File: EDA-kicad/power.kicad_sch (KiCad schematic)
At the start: 93 parts, among them SW1 EG25-switch-CSS-1210MC, SW2 MIC-switch-CSS-1210MC, SW3 CAM-switch-CSS-1210MC, U10 22V-boost-AP3032KTR-G1, U11 MP3429GL-Z, U7 BQ25792RQMR, U8 TPS65023BRSBR, U9 BAT-CONNECTOR-FLTS22WR00

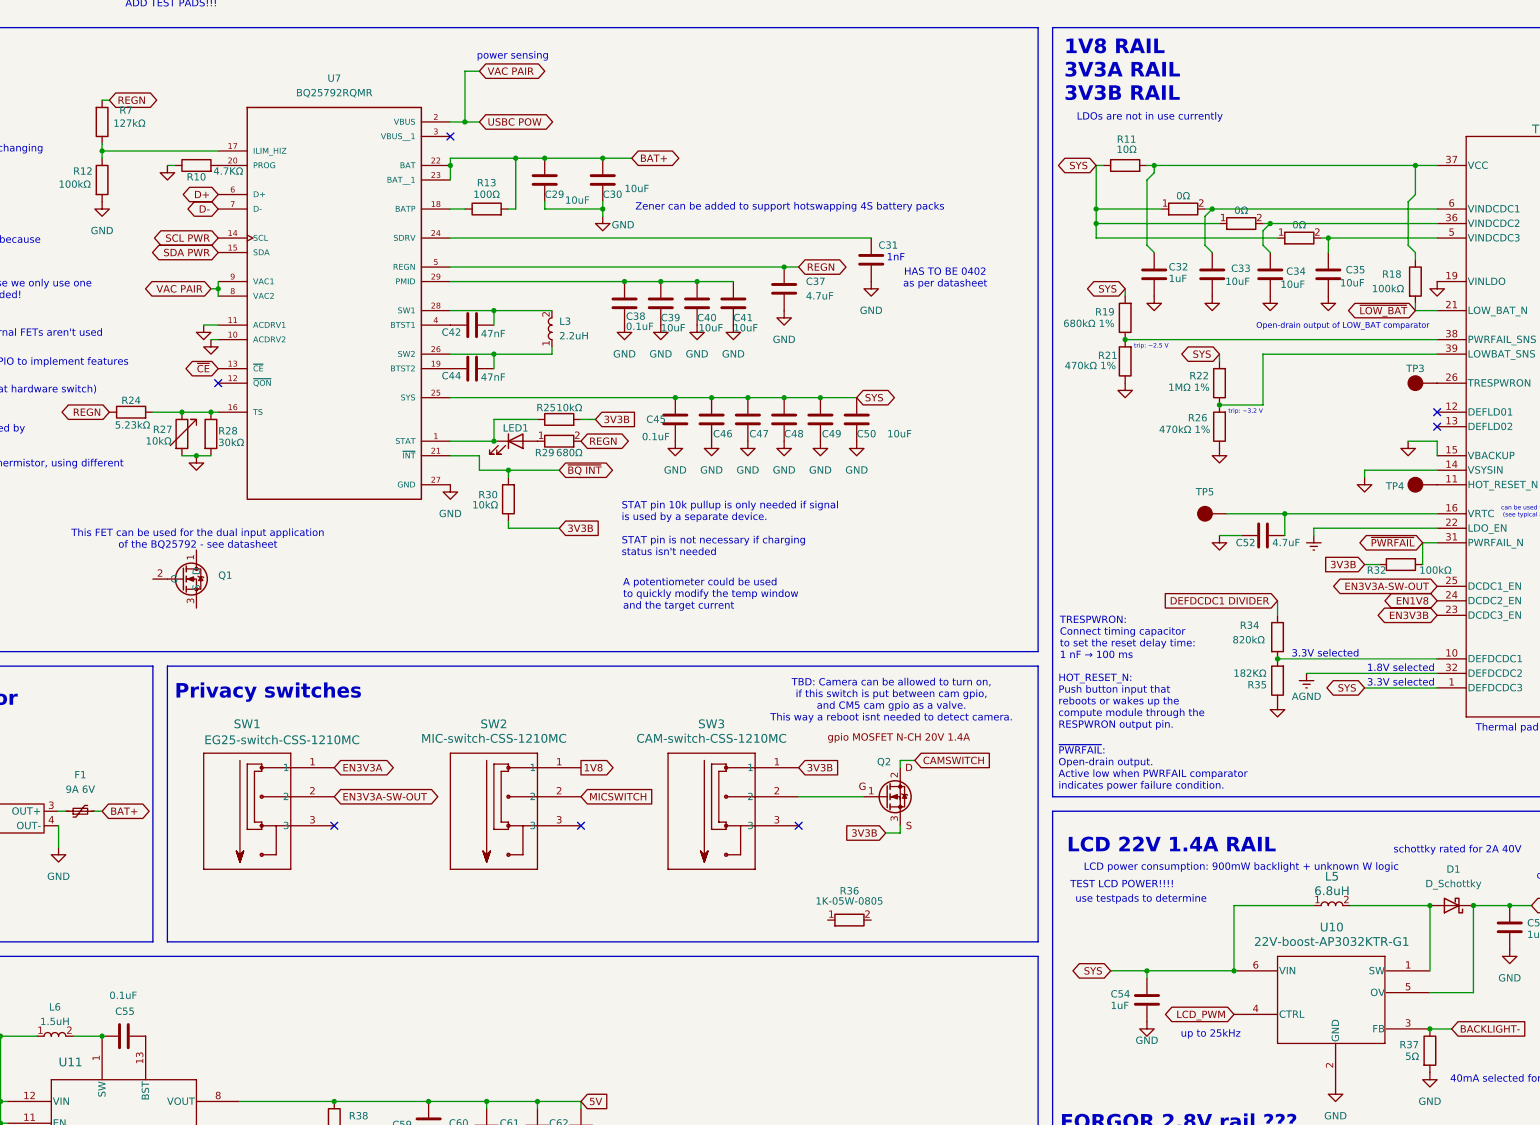
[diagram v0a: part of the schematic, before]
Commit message: change some labels
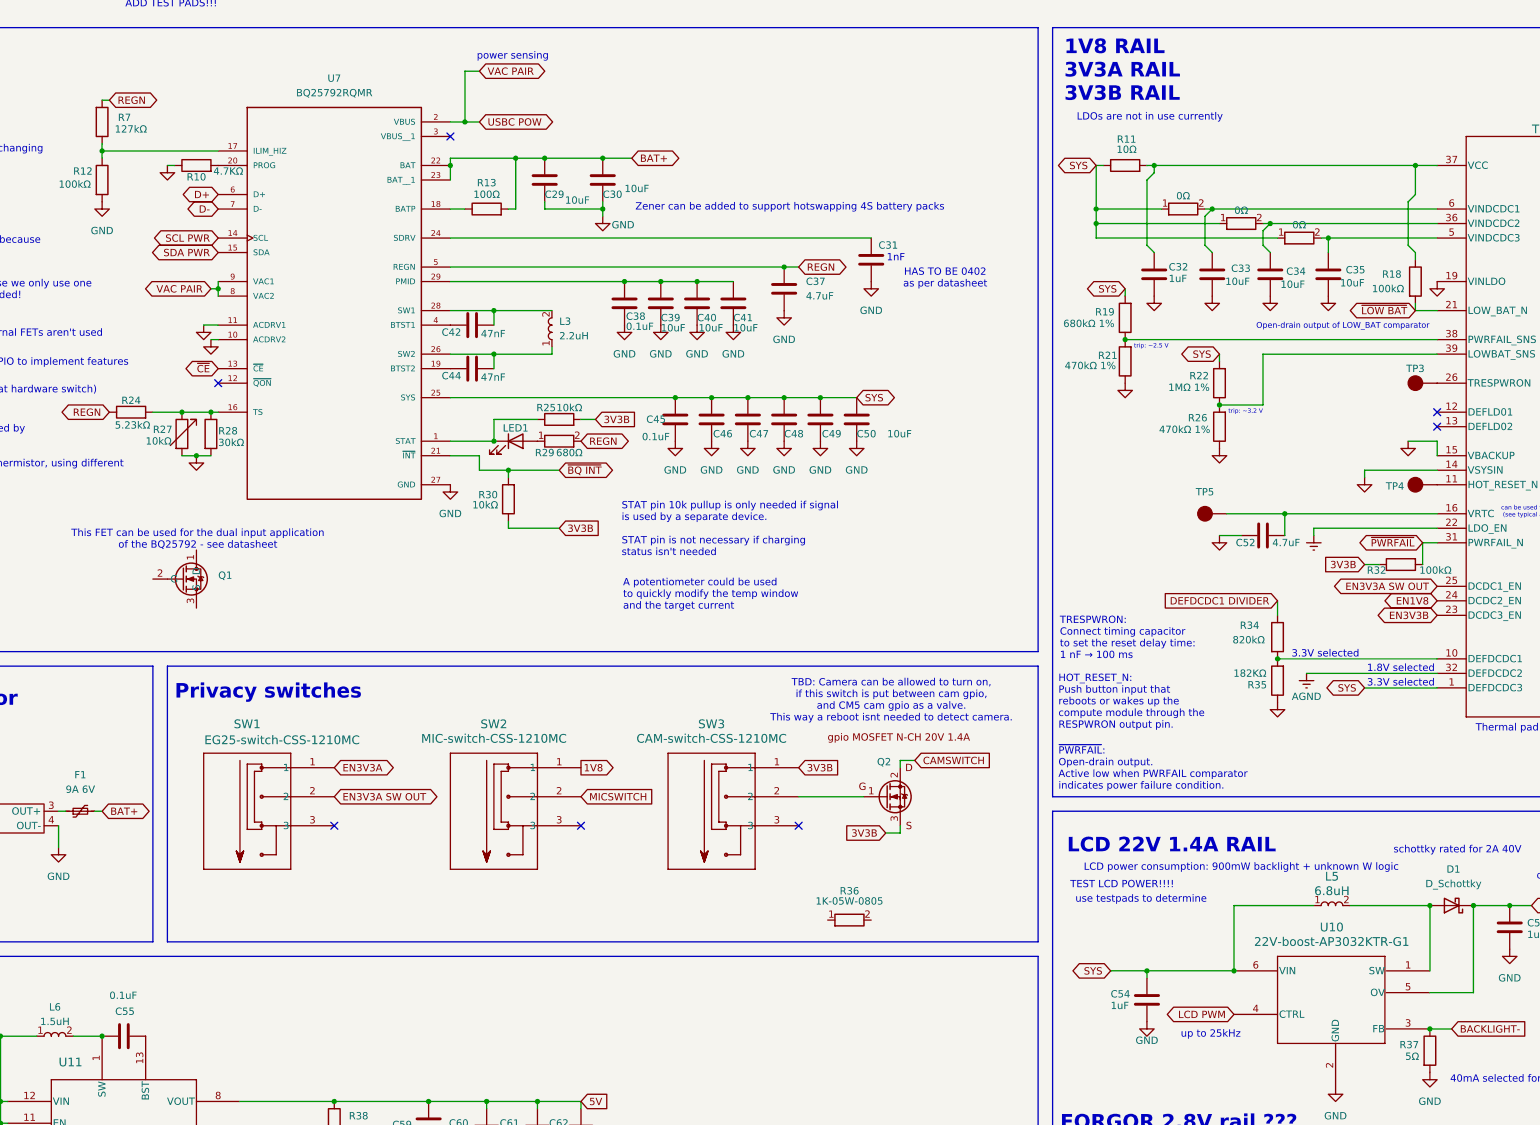
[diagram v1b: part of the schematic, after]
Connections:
- net EN3V3A-SW-OUT renamed EN3V3A SW OUT
- net LCD_PWM renamed LCD PWM
- net ~{LOW_BAT} renamed ~{LOW BAT}
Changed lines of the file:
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@@
 		)
 	)
-	(global_label "LCD_PWM"
+	(global_label "LCD PWM"
 		(shape bidirectional)
 		(at 267.97 223.52 180)
@@
 		)
 	)
-	(global_label "~{LOW_BAT}"
+	(global_label "~{LOW BAT}"
 		(shape bidirectional)
 		(at 299.72 100.33 180)
@@
 		)
 	)
-	(global_label "EN3V3A-SW-OUT"
+	(global_label "EN3V3A SW OUT"
 		(shape bidirectional)
 		(at 303.53 148.59 180)
@@
 		)
 		(property "Intersheetrefs" "${INTERSHEET_REFS}"
-			(at 282.9235 148.59 0)
+			(at 284.1331 148.59 0)
 			(effects
 				(font
@@
 		)
 	)
-	(global_label "EN3V3A-SW-OUT"
+	(global_label "EN3V3A SW OUT"
 		(shape bidirectional)
 		(at 110.49 185.42 0)
@@
 		)
 		(property "Intersheetrefs" "${INTERSHEET_REFS}"
-			(at 131.0965 185.42 0)
+			(at 129.8869 185.42 0)
 			(effects
 				(font
@@
 		(dnp no)
 		(property "Reference" "R7"
-			(at 75.184 65.278 0)
+			(at 74.93 66.548 0)
 			(effects
 				(font
@@
 		)
 		(property "Value" "127kΩ"
-			(at 77.47 67.564 0)
+			(at 77.724 68.58 0)
 			(effects
 				(font
